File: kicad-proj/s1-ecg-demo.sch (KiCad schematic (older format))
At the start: 58 parts, among them J1 Left arm, J2 Right arm, J3 Right leg, J4 USB-C-16-Pin, J5 TC2030, J6 Current Probe, J7 Battery Port, U1 AD8233

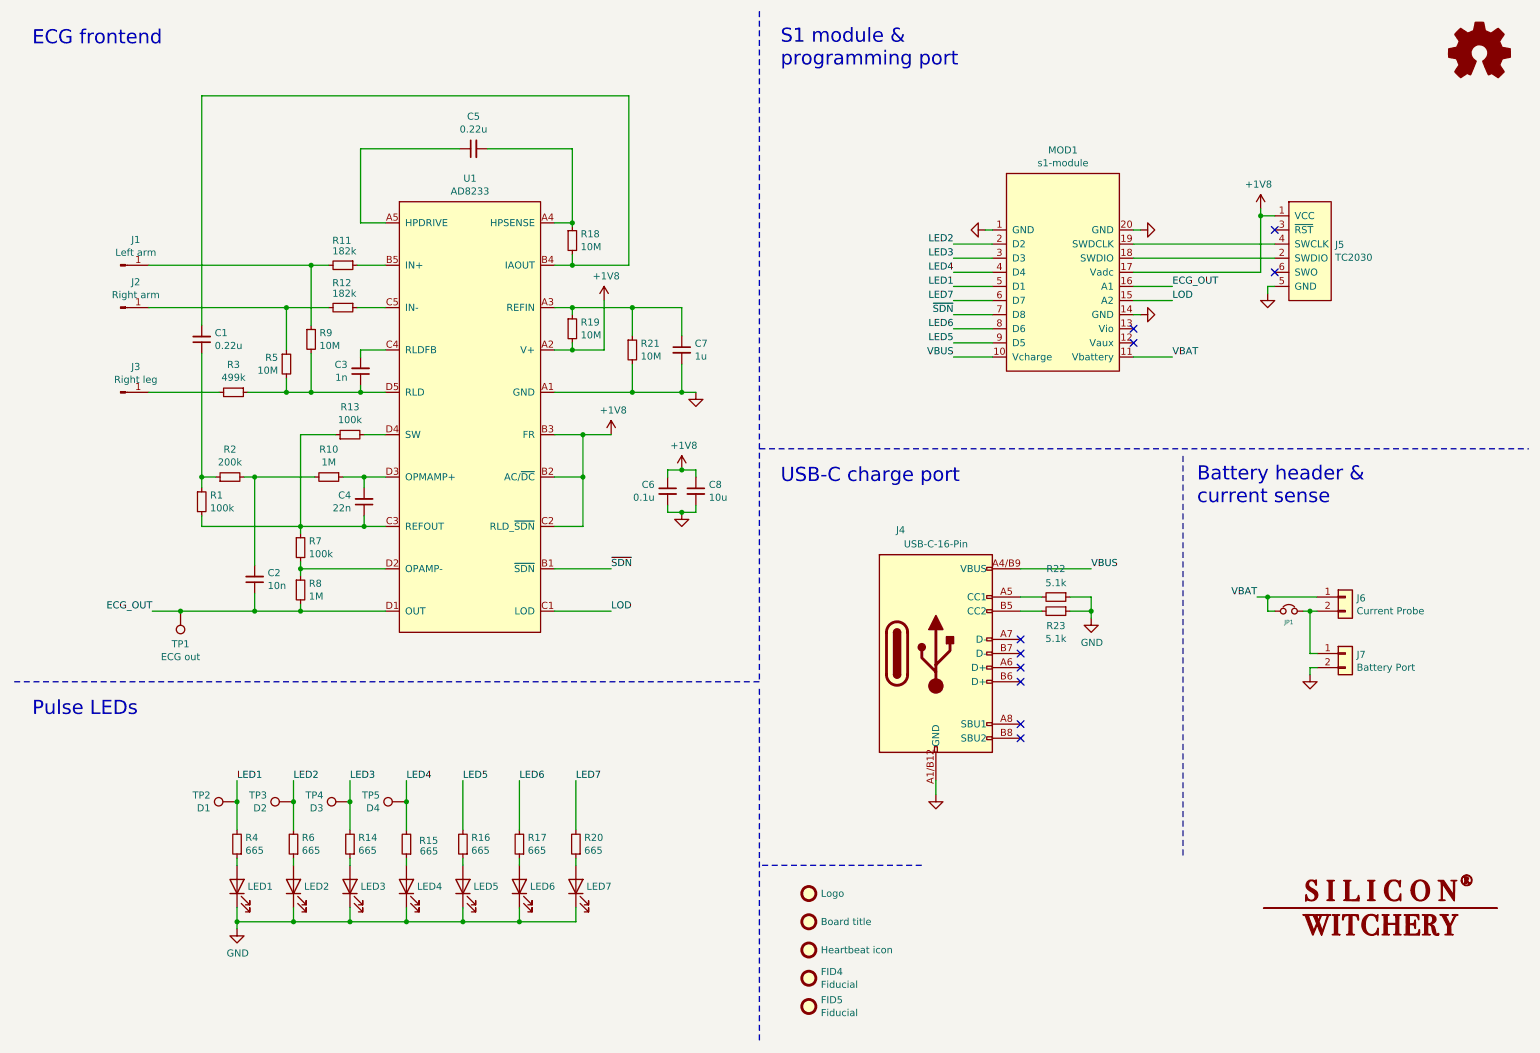
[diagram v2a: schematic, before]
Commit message: Little bit of clean up fixed battery and current header re-exported gerbers
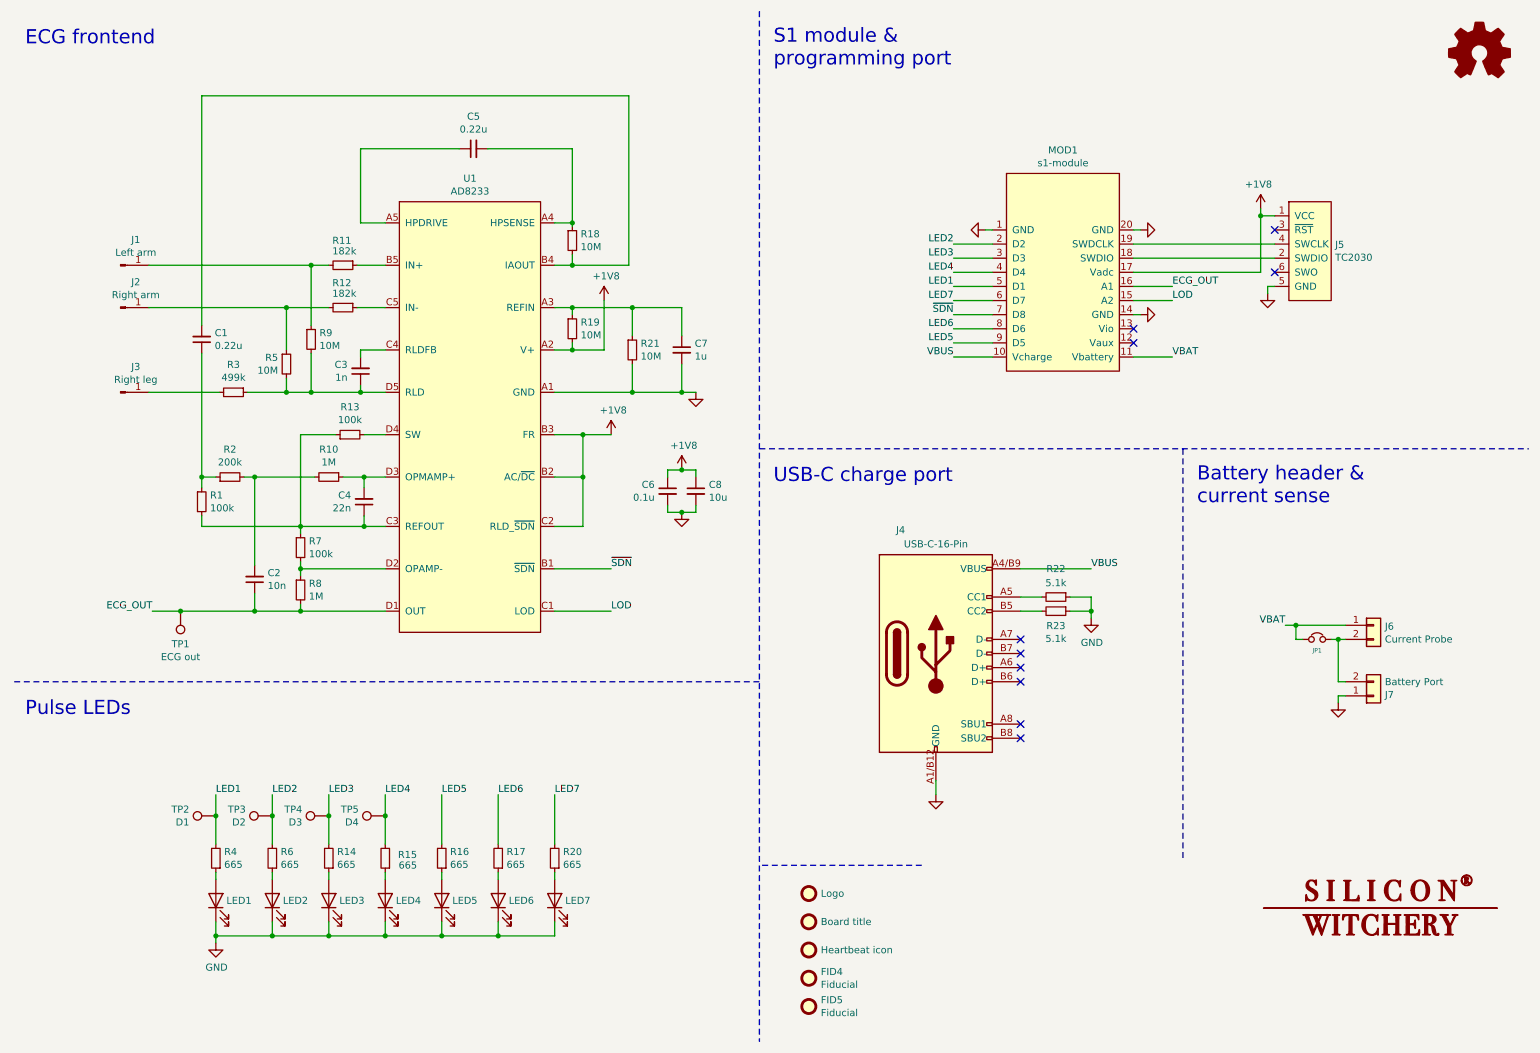
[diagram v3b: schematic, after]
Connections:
- net GND: now also J7.1 (Pin_1); no longer J7.2 (Pin_2)
- net at J6.2 (Pin_2), JP1.1: now also J7.2 (Pin_2); no longer J7.1 (Pin_1)
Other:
- moved on the sheet: J6, J7, JP1, LED1, LED2, LED3, LED4, LED5, LED6, LED7, R14, R15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
